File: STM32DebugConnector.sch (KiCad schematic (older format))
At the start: 12 parts, among them J1 USB_B_Micro, J2 STM32_Debug, J3 STDC32, SW1 RESET, U1 NJM2884U1

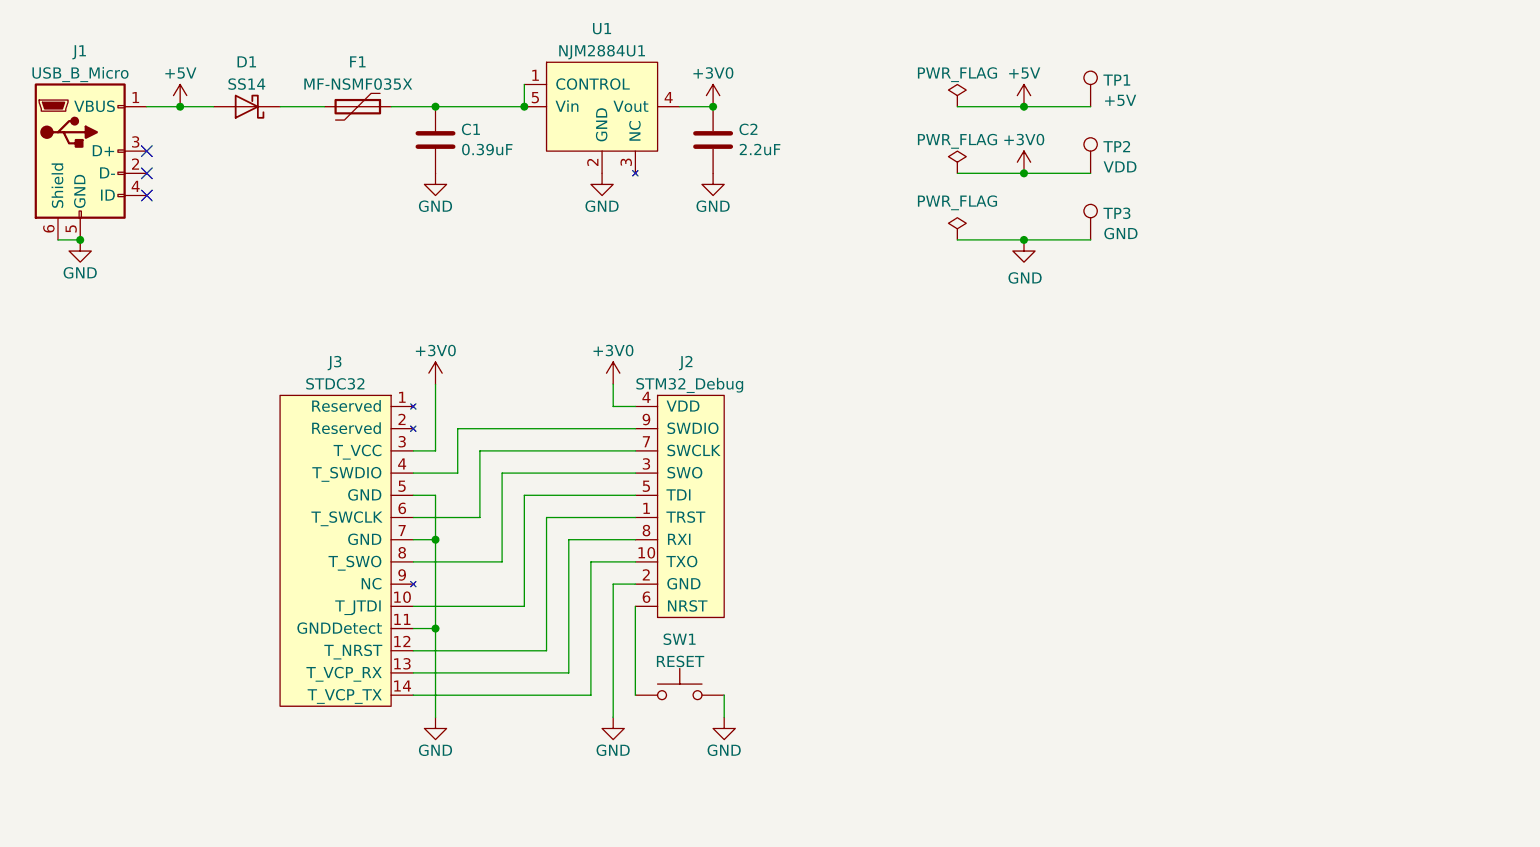
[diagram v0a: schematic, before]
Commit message: 基板 V2.0
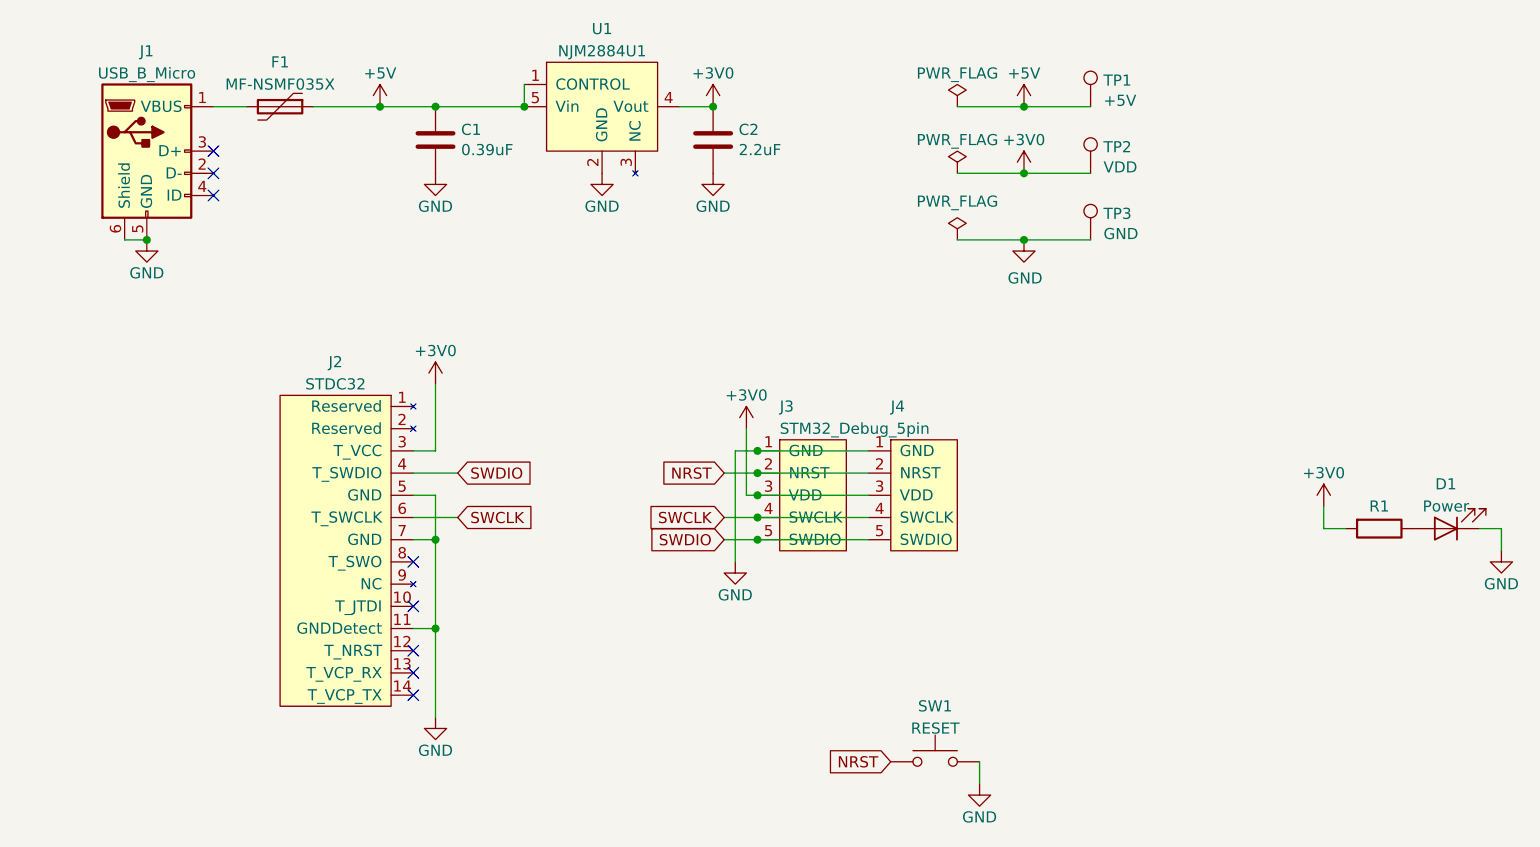
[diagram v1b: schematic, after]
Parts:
- removed D1: SS14, Diode_SMD:D_SMA_Handsoldering, symbol Device:D_Schottky
- removed J2: STM32_Debug, Connector_PinSocket_1.27mm:PinSocket_2x05_P1.27mm_Vertical, symbol STM32DebugConnector:STM32_Debug
- added D1: Power, LED_SMD:LED_0603_1608Metric_Pad1.05x0.95mm_HandSolder, symbol Device:LED
- added J3, J4: STM32_Debug_5pin, STM32DebugConnector:STM32_Debug_5pin, symbol STM32DebugConnector:STM32_Debug_5pin
- added R1: R, Resistor_SMD:R_0603_1608Metric_Pad1.05x0.95mm_HandSolder, symbol Device:R
- U1: footprint Package_TO_SOT_SMD:SOT-89-5_Handsoldering -> Package_TO_SOT_SMD:SOT-89-5
- renumbered J3 to J2
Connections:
- net +3V0: now also J3.3 (VDD), J4.3 (VDD), R1.2
- net +5V: now also C1.1, F1.1, U1.1 (CONTROL), U1.5 (Vin); no longer J1.1 (VBUS)
- net GND: now also D1.1 (K), J3.1 (GND), J4.1 (GND)
- net SWDIO: now reaches J2.4 (T_SWDIO)
- net SWDIO: now also J3.5 (SWDIO), J4.5 (SWDIO)
- net SWCLK: now reaches J2.6 (T_SWCLK)
- net SWCLK: now also J3.4 (SWCLK), J4.4 (SWCLK)
- net at F1.2: now also J1.1 (VBUS)
- net NRST: now reaches SW1.1
- net NRST: now also J3.2 (NRST), J4.2 (NRST)
- new net: D1.2 (A), R1.1
- no-connect marks 3 -> 8
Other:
- moved on the sheet: F1, J1, SW1
